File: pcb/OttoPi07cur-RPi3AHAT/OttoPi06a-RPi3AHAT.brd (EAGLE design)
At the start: 56 x 65 mm, 36 parts

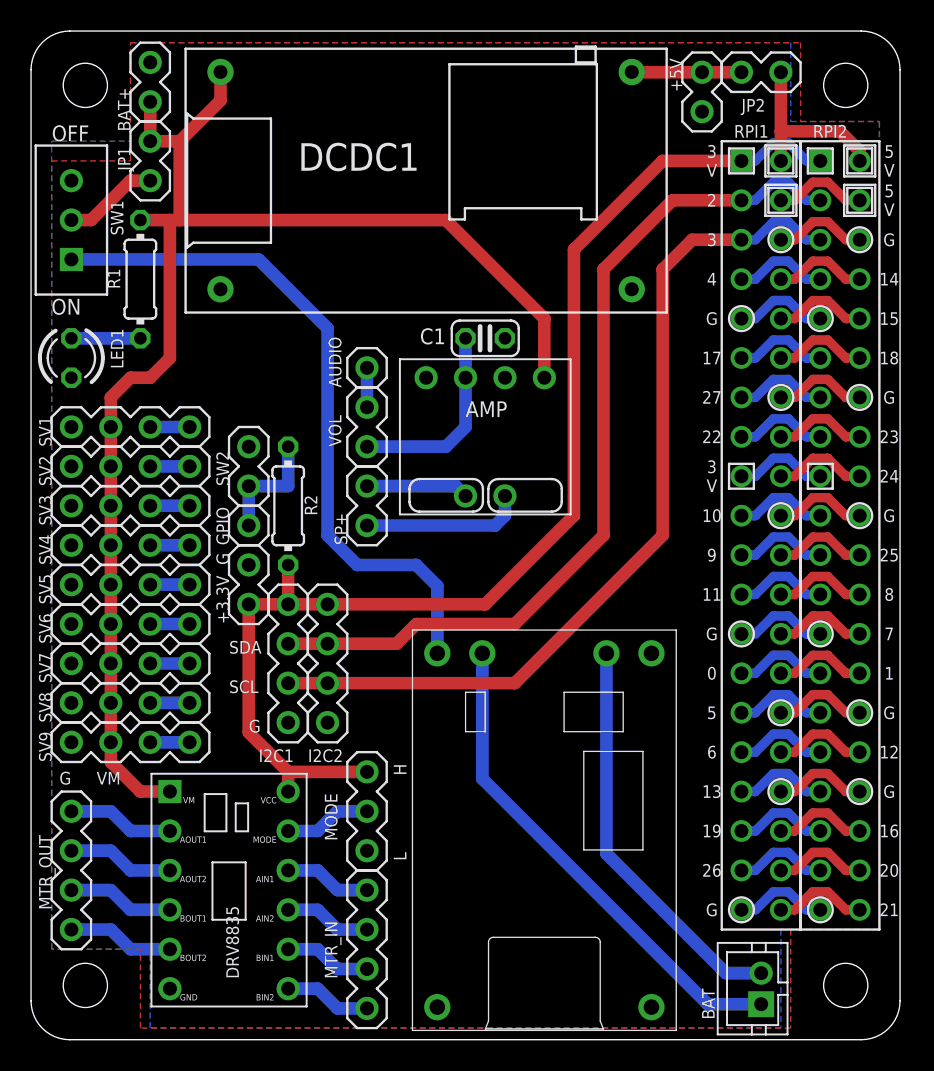
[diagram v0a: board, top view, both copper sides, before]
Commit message: [update] PCB
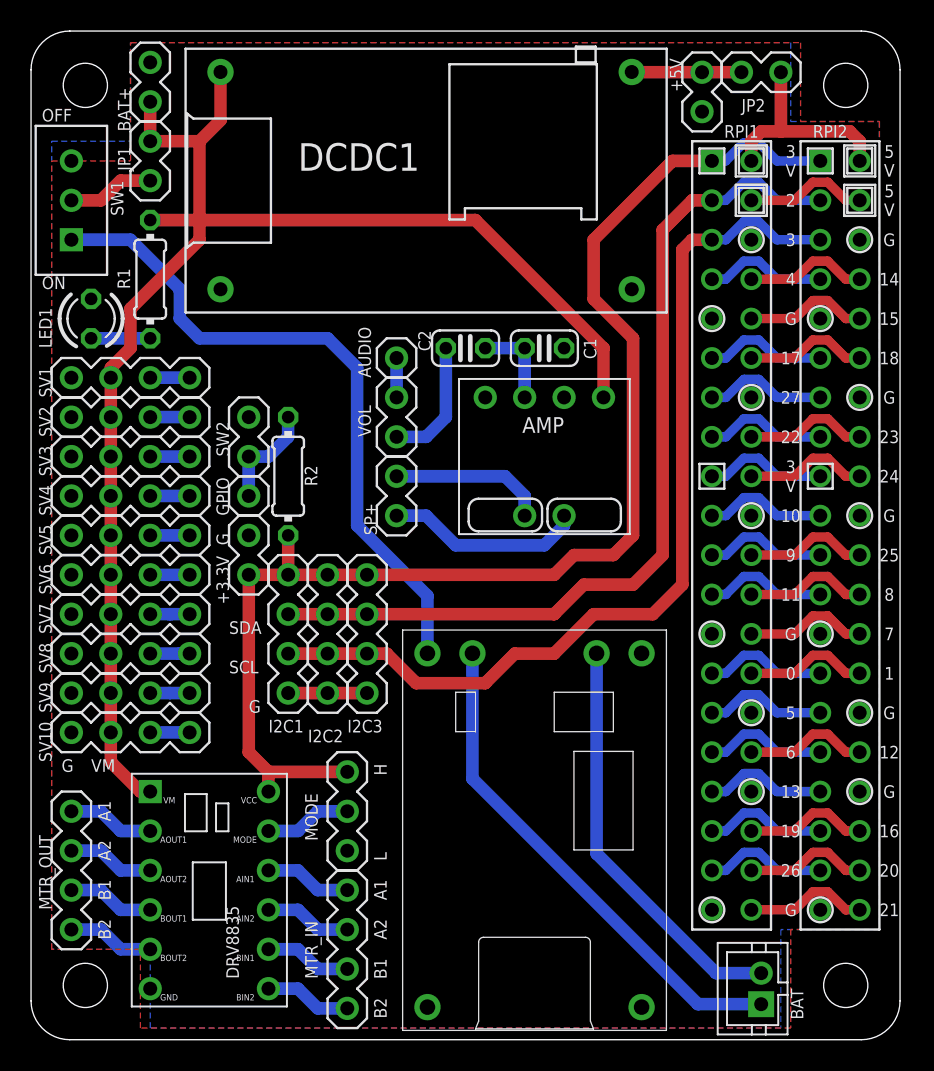
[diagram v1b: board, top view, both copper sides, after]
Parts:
- added C2: 0.1uF, rcl:C025-024X044
- added I2C3, SV10: (no value), ytani1:PINHEAD-MA04-1
- moved AMP 4.02 mm to (5.08, 5.08)
- moved C1 3.86 mm to (5.08, 12.1)
- moved SV7 3.18 mm to (-21.6, -5.08)
- moved SV9 3.18 mm to (-21.6, -10.2)
- moved SV1 3.17 mm to (-21.6, 10.2)
- moved SV2 3.17 mm to (-21.6, 7.62)
- moved SV3 3.17 mm to (-21.6, 5.08)
- moved SV4 3.17 mm to (-21.6, 2.54)
- moved SV5 3.17 mm to (-21.6, 0.00)
- moved SV6 3.17 mm to (-21.6, -2.54)
- moved SV8 3.17 mm to (-21.6, -7.62)
- moved LED1 2.84 mm to (-24.1, 14.0), turned to 90 degrees
- moved AUDIO 2.01 mm to (-5.71, 11.4)
- moved SP+ 2.01 mm to (-4.45, 2.54)
- moved VOL 2.01 mm to (-4.45, 7.62)
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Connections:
- new net N$15: C2.2, VOL.1
- new net N$17: SV10.3, SV10.4
- net +3V3: now also I2C3.1
- net AUDIO1: now also C2.1; no longer VOL.1
- net BAT+: now also SV10.2
- net GND: now also I2C3.4, SV10.1
- net SCL: now also I2C3.3
- net SDA: now also I2C3.2
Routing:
- net GND: track 48.3 -> 5.08 mm
- net N$15: track 0.00 -> 8.15 mm
- net AUDIO1: track 12.6 -> 5.71 mm
- net +3V3: track 80.4 -> 85.7 mm
- net SP-: track 6.61 -> 10.1 mm
- net SCL: track 57.1 -> 60.5 mm
- net BAT+: track 89.4 -> 92.2 mm
- net N$17: track 0.00 -> 2.54 mm
- net SP+: track 10.4 -> 12.7 mm
- net N$6: track 12.0 -> 13.9 mm
- net N$39: track 6.04 -> 7.95 mm
- net N$38: track 6.04 -> 7.95 mm
- net N$36: track 6.04 -> 7.95 mm
- net N$33: track 6.04 -> 7.95 mm
- net N$30: track 6.04 -> 7.95 mm
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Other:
- board text added: "A1"
- board text added: "A2"
- board text added: "B1"
- board text added: "B2"
